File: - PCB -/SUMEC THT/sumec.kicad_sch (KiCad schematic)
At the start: 0 parts

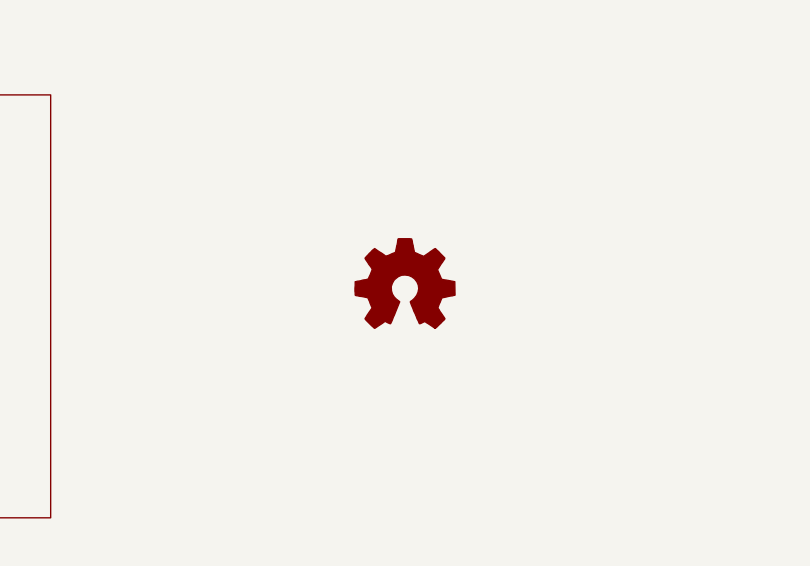
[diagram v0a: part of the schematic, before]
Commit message: QRE Array - WIP
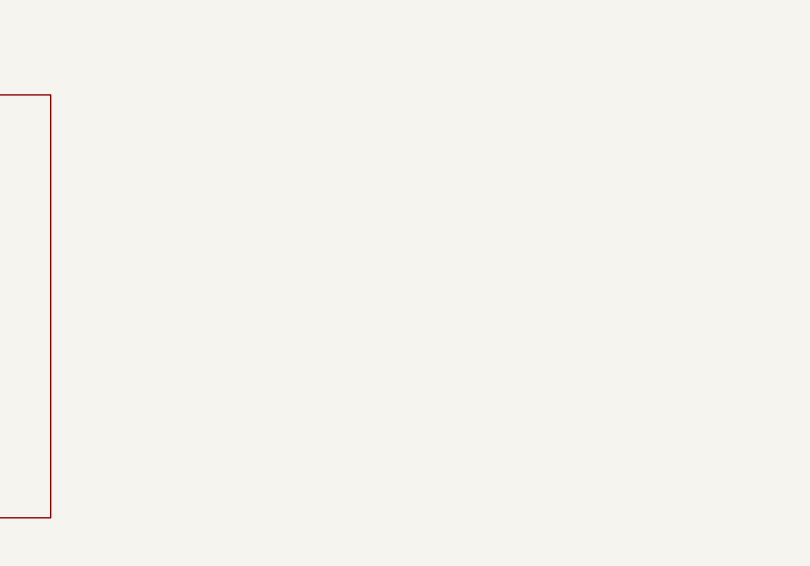
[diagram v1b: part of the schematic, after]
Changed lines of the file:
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@@
     (company "SPŠ NA PROSEKU")
-  )
-  (symbol (lib_id "Graphic:Logo_Open_Hardware_Small") (at 130.81 105.41 0) (unit 1)
-    (in_bom no) (on_board no) (dnp no) (fields_autoplaced)
-    (property "Reference" "#SYM1" (at 130.81 98.425 0)
-      (effects (font (size 1.27 1.27)) hide)
-    )
-    (property "Value" "Logo_Open_Hardware_Small" (at 130.81 111.125 0)
-      (effects (font (size 1.27 1.27)) hide)
-    )
-    (property "Footprint" "" (at 130.81 105.41 0)
-      (effects (font (size 1.27 1.27)) hide)
-    )
-    (property "Datasheet" "~" (at 130.81 105.41 0)
-      (effects (font (size 1.27 1.27)) hide)
-    )
-    (property "Sim.Enable" "0" (at 130.81 105.41 0)
-      (effects (font (size 1.27 1.27)) hide)
-    )
-    (instances
-      (project "sumec"
-        (path "/fc70a1a8-ed7c-4a0f-9b1a-f23293528385"
-          (reference "#SYM1") (unit 1)
-        )
-      )
-    )
   )
   (sheet (at 21.59 83.82) (size 69.85 46.99)
